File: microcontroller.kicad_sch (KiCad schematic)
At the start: 21 parts, among them J1 SWD, SW1 RESET, U1 STM32F103C8Tx, Y1 8MHz

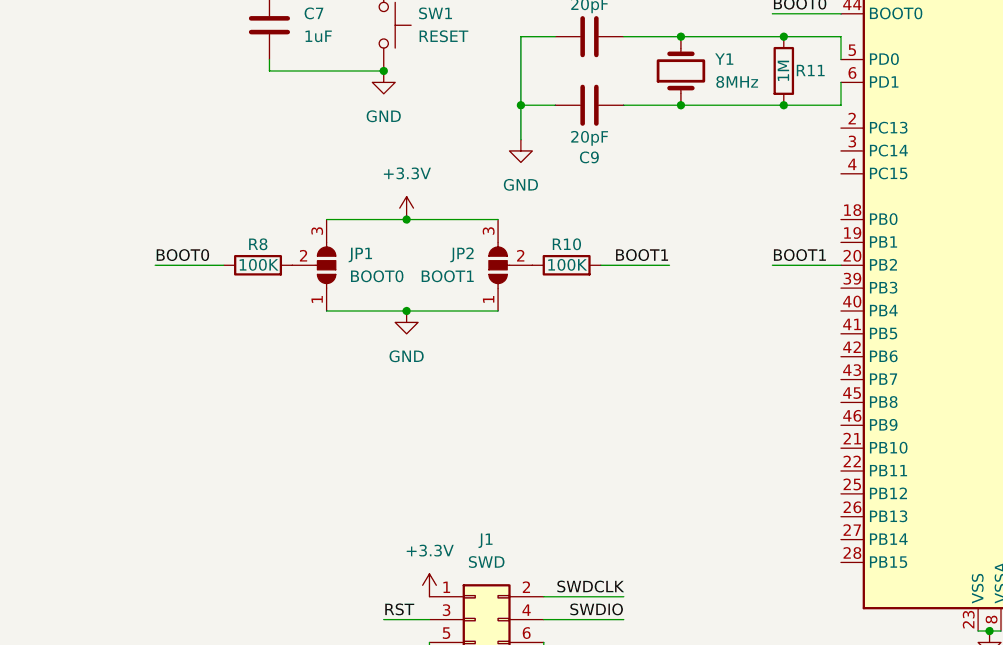
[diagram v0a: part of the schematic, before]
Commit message: i2c
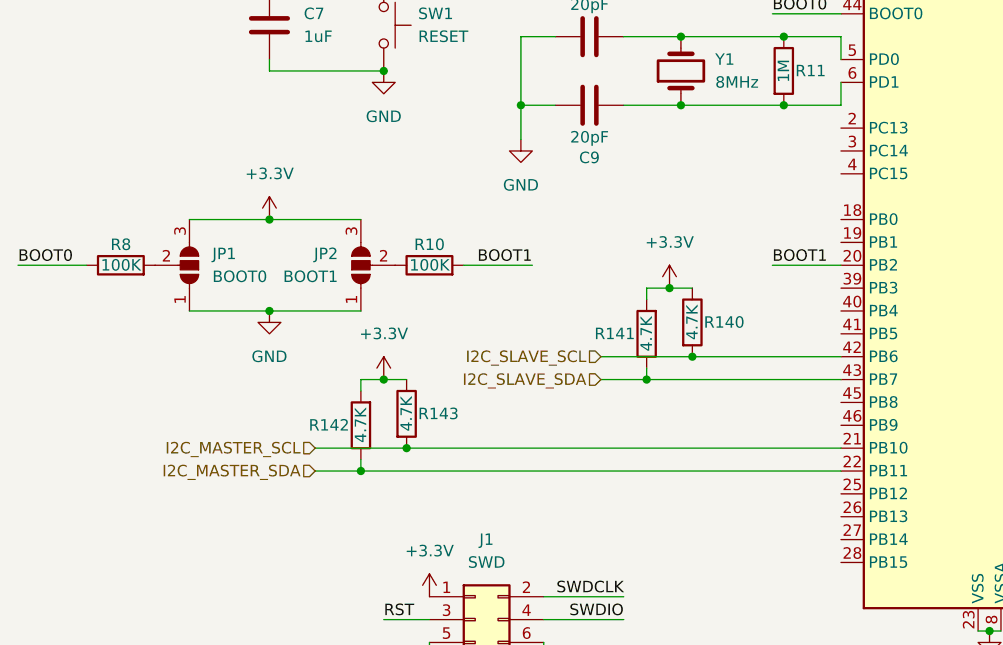
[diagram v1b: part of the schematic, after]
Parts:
- added R140, R141, R142, R143: 4.7K, symbol Device:R
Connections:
- net +3.3V: now also R140.1, R141.2, R142.2, R143.1
- net I2C_MASTER_SCL: now reaches U1.21 (PB10)
- net I2C_MASTER_SCL: now also R143.2
- net I2C_MASTER_SDA: now reaches U1.22 (PB11)
- net I2C_MASTER_SDA: now also R142.1
- net I2C_SLAVE_SCL: now reaches U1.42 (PB6)
- net I2C_SLAVE_SCL: now also R140.2
- net I2C_SLAVE_SDA: now reaches U1.43 (PB7)
- net I2C_SLAVE_SDA: now also R141.1
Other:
- moved on the sheet: JP1, JP2, R10, R8
